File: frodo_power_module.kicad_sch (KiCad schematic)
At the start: 61 parts, among them J1 Keystone 1098, J10 SWD Header, J2 Molex MicroFit 2x2, J3 Molex MicroFit 2x2, J4 Molex MicroFit 2x2, J5 Molex MicroFit 2x2, J6 Molex MicroFit 2x2, J7 JST-GH, J8 JST-GH, J9 JST-GH, U1 STM32F042F6Px, U2 L7805, U3 AZ1117I-3.3, U4 BQ25171-Q1, U5 BQ29200, U6 MCP2562-E-SN, Y1 8MHz

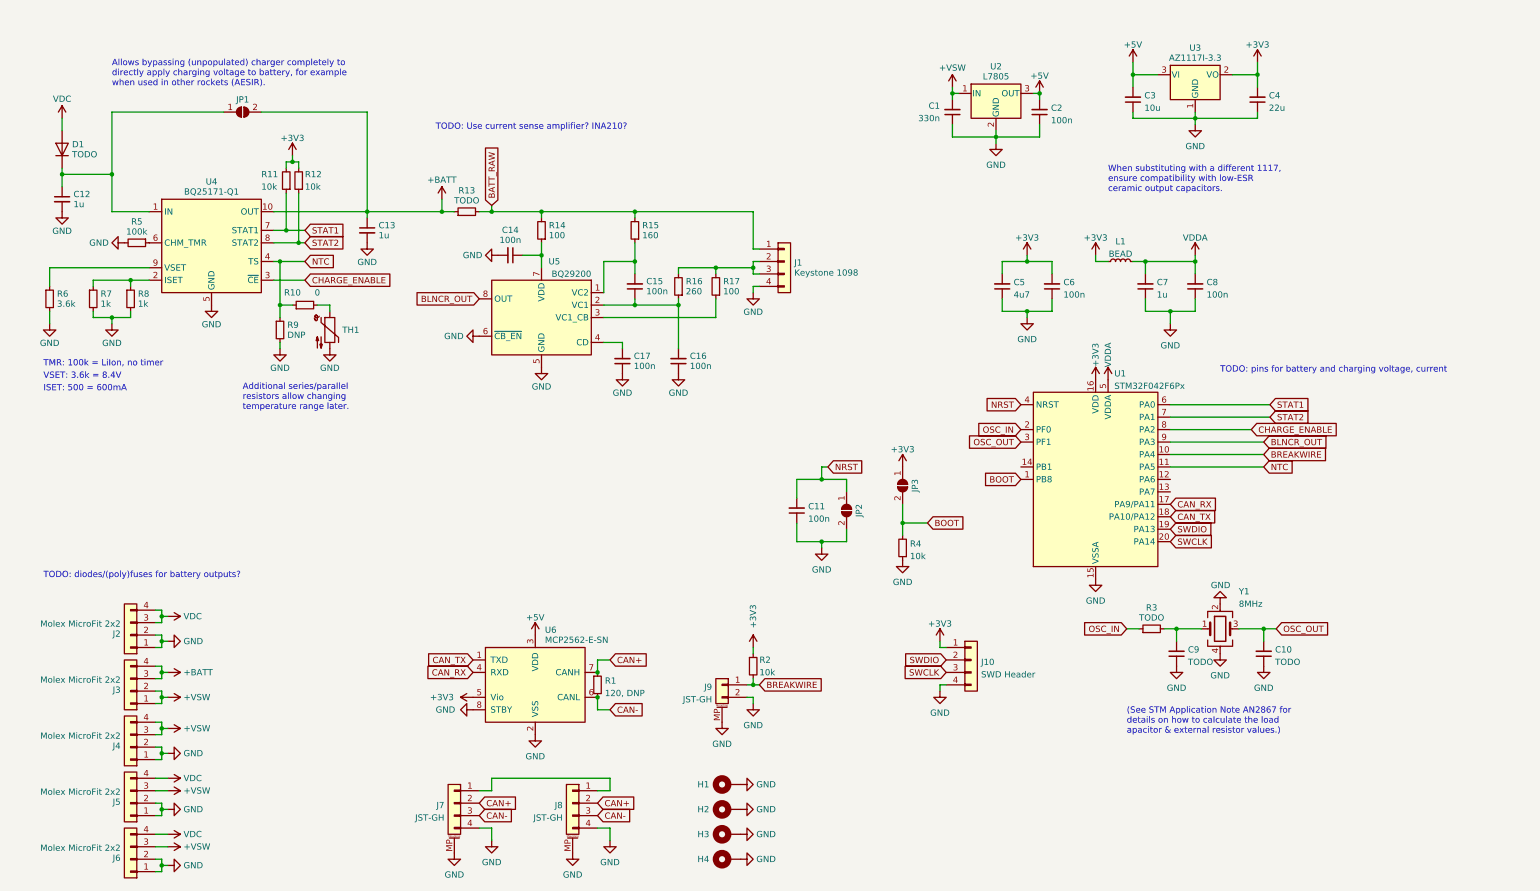
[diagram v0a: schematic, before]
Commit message: Add current sense amp to PCB
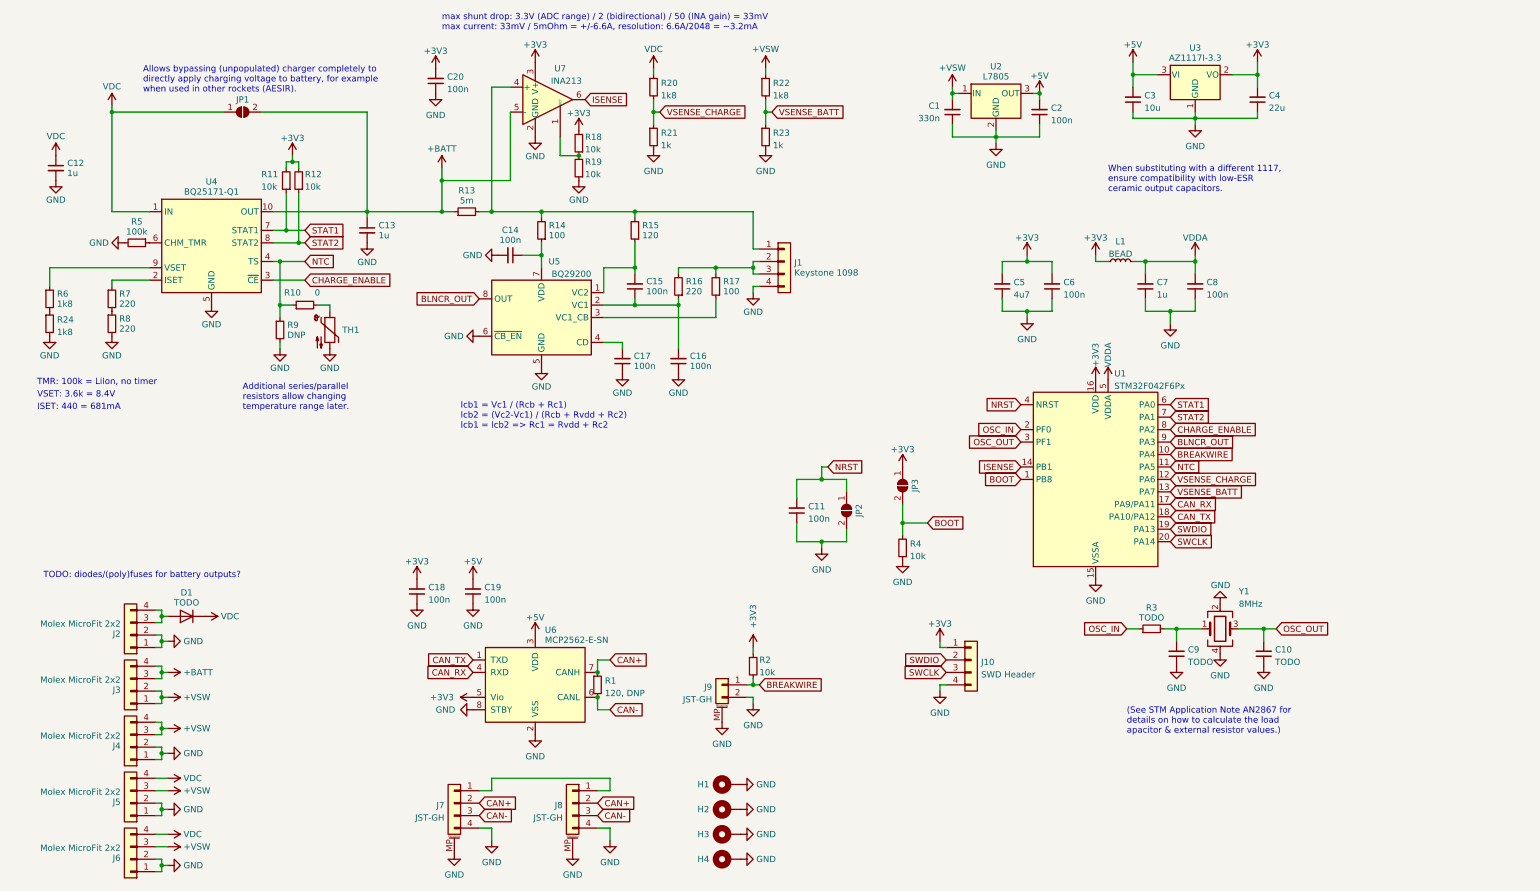
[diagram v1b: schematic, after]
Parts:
- added C18, C19, C20: 100n, Capacitor_SMD:C_0603_1608Metric, symbol Device:C_Small
- added R18, R19: 10k, Resistor_SMD:R_0603_1608Metric, symbol Device:R_Small
- added R20, R22, R24: 1k8, Resistor_SMD:R_0603_1608Metric, symbol Device:R_Small
- added R21, R23: 1k, Resistor_SMD:R_0603_1608Metric, symbol Device:R_Small
- added U7: INA213, Package_TO_SOT_SMD:SOT-363_SC-70-6, symbol frodo_power_module:INA210
- R10, R14, R17: LCSC# C98220 -> (none); Part# RC0603FR-0710KL -> (none)
- R13: value TODO -> 5m
- R15: value 160 -> 120; LCSC# C98220 -> C114640; Part# RC0603FR-0710KL -> RC0603FR-07120RL
- R16: value 260 -> 220
- R2: LCSC# C114640 -> C98220; Part# RC0603FR-07120RL -> RC0603FR-0710KL
- R6: value 3.6k -> 1k8; LCSC# C98220 -> C185354; Part# RC0603FR-0710KL -> RC0603FR-071K8L
- R7, R8: value 1k -> 220
- R9: LCSC# C98220 -> (none); Manufacturer YAGEO -> (none); Part# RC0603FR-0710KL -> (none)
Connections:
- net +3V3: now also C18.2, C20.2, R18.2, U7.3 (V+)
- net +5V: now also C19.2
- net +BATT: now also U7.5 (-)
- net +VSW: now also R22.1
- net GND: now also C18.1, C19.1, C20.1, R19.1, R21.2, R23.2, R24.2, U7.2 (GND); no longer R6.2, R7.2
- net VDC: now also C12.1, D1.1 (K), JP1.1 (A), U4.1 (IN), R20.1; no longer D1.2 (A), J2.3 (Pin_3), J2.4 (Pin_4)
- net at R7.1, U4.2 (ISET): no longer R8.1
- net VSENSE_CHARGE: now reaches U1.12 (PA6)
- net VSENSE_CHARGE: now also R20.2, R21.1
- net VSENSE_BATT: now reaches U1.13 (PA7)
- net VSENSE_BATT: now also R22.2, R23.1
- net ISENSE: now reaches U1.14 (PB1)
- net ISENSE: now also U7.6
- net BATT_RAW: no longer names the net of J1.1 (Pin_1), R13.2, R14.2, R15.2
- net BATT_RAW: now also U7.4 (+)
- new net: R18.1, R19.2, U7.1 (REF)
- new net: R24.1, R6.2
- new net: R7.2, R8.1
- new net: D1.2 (A), J2.3 (Pin_3), J2.4 (Pin_4)
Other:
- note added: "ISET: 440 = 681mA"
- note added: "Icb1 = Vc1 / (Rcb + Rc1) Icb2 = (Vc2-Vc1) / (Rcb + Rvdd + Rc2) Icb1 = Icb2 => Rc1 = Rvdd + Rc2"
- note added: "max shunt drop: 3.3V (ADC range) / 2 (bidirectional) / 50 (INA gain) = 33mV max current: 33mV / 5mOhm = +/-6.6A, resolution: 6.6A/2048 = ~3.2mA"
- note removed: "ISET: 500 = 600mA"
- note removed: "TODO: Use current sense amplifier? INA210?"
- note removed: "TODO: pins for battery and charging voltage, current"
- moved on the sheet: C12, D1, R7, R8
